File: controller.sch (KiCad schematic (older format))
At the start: 21 parts, among them J2 UART, J3 programming header, J4 Micro_SD_Card_Det, SW2 RAM~FLASH, SW3 start, SW4 stop, SW5 Rotary_Encoder_Switch, U1 WM8778-units, U5 STM32F401RC, U6 lcd, Y1 CSTLS4M00G53-B0

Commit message: ksch: change component values to include the unit except for resistors add more info to some devices
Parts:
- C31: value 4.7u -> 4.7uF
- C32: value 10u -> 10uF
- C33: value 0.1u -> 100nF
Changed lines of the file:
@@
 Sheet 3 4
 Title "OpenLoop"
-Date "2017-09-25"
+Date "2017-10-02"
 Rev "A"
 Comp ""
@@
 P 8900 5600
 F 0 "C33" H 8992 5646 50  0000 L CNN
-F 1 "0.1u" H 8992 5555 50  0000 L CNN
+F 1 "100nF" H 8992 5555 50  0000 L CNN
 F 2 "Capacitors_SMD:C_0805_HandSoldering" H 8900 5600 50  0001 C CNN
 F 3 "" H 8900 5600 50  0001 C CNN
@@
 P 7950 6150
 F 0 "C32" H 8100 6100 50  0000 R CNN
-F 1 "10u" H 8150 6200 50  0000 R CNN
+F 1 "10uF" H 8150 6200 50  0000 R CNN
 F 2 "Capacitors_SMD:C_0805_HandSoldering" H 7950 6150 50  0001 C CNN
 F 3 "" H 7950 6150 50  0001 C CNN
@@
 P 6950 4250
 F 0 "C31" H 7100 4200 50  0000 R CNN
-F 1 "4.7u" H 7150 4300 50  0000 R CNN
+F 1 "4.7uF" H 7150 4300 50  0000 R CNN
 F 2 "Capacitors_SMD:C_0805_HandSoldering" H 6950 4250 50  0001 C CNN
 F 3 "" H 6950 4250 50  0001 C CNN

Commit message: migrate to kicad v5
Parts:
- C31, C32, C33: symbol C_Small -> Device:C_Small
- J2: symbol CONN_01X02 -> Connector:Conn_01x02_Male
- J3: symbol CONN_01X04 -> Connector:Conn_01x04_Male
- J4: symbol Micro_SD_Card_Det -> Connector:Micro_SD_Card_Det
- R4, R5, R6, R7: symbol R_Small -> Device:R_Small
- RV1, RV2, RV3: symbol POT -> Device:R_POT
- SW2: symbol SW_SPDT -> Switch:SW_SPDT
- SW3, SW4: symbol SW_Push -> Switch:SW_Push
- SW5: symbol Rotary_Encoder_Switch -> Device:Rotary_Encoder_Switch
- U1: symbol WM8778-units -> openloop:WM8778-units
- U5: symbol STM32F401RC -> openloop:STM32F401RC
- U6: symbol lcd -> openloop:lcd
- Y1: symbol Resonator_Small -> Device:Resonator_Small
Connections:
- wire segments 60 -> 73
- no-connect marks 0 -> 21

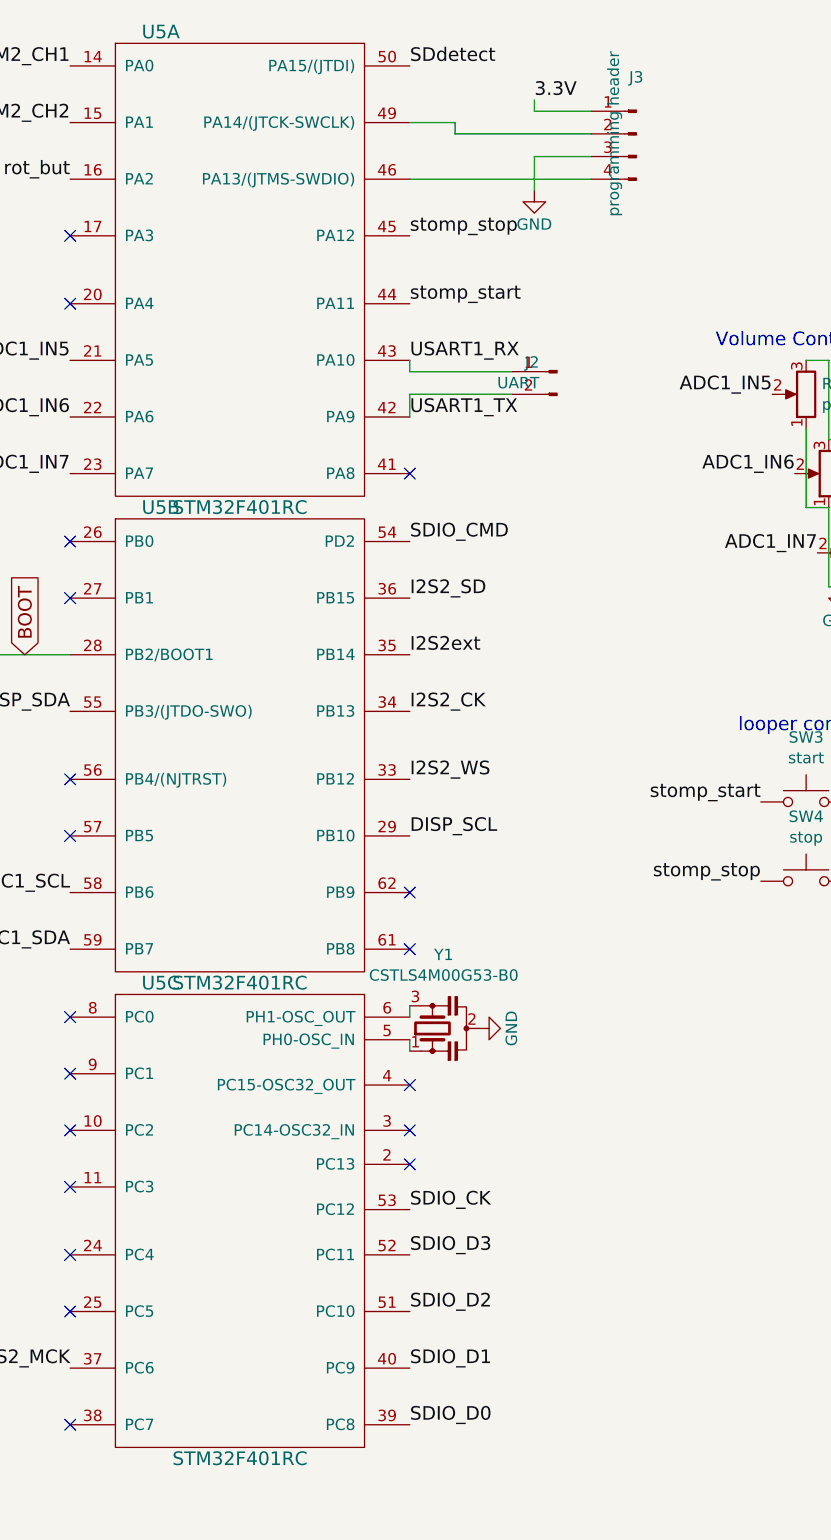
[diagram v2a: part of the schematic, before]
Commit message: ready for print
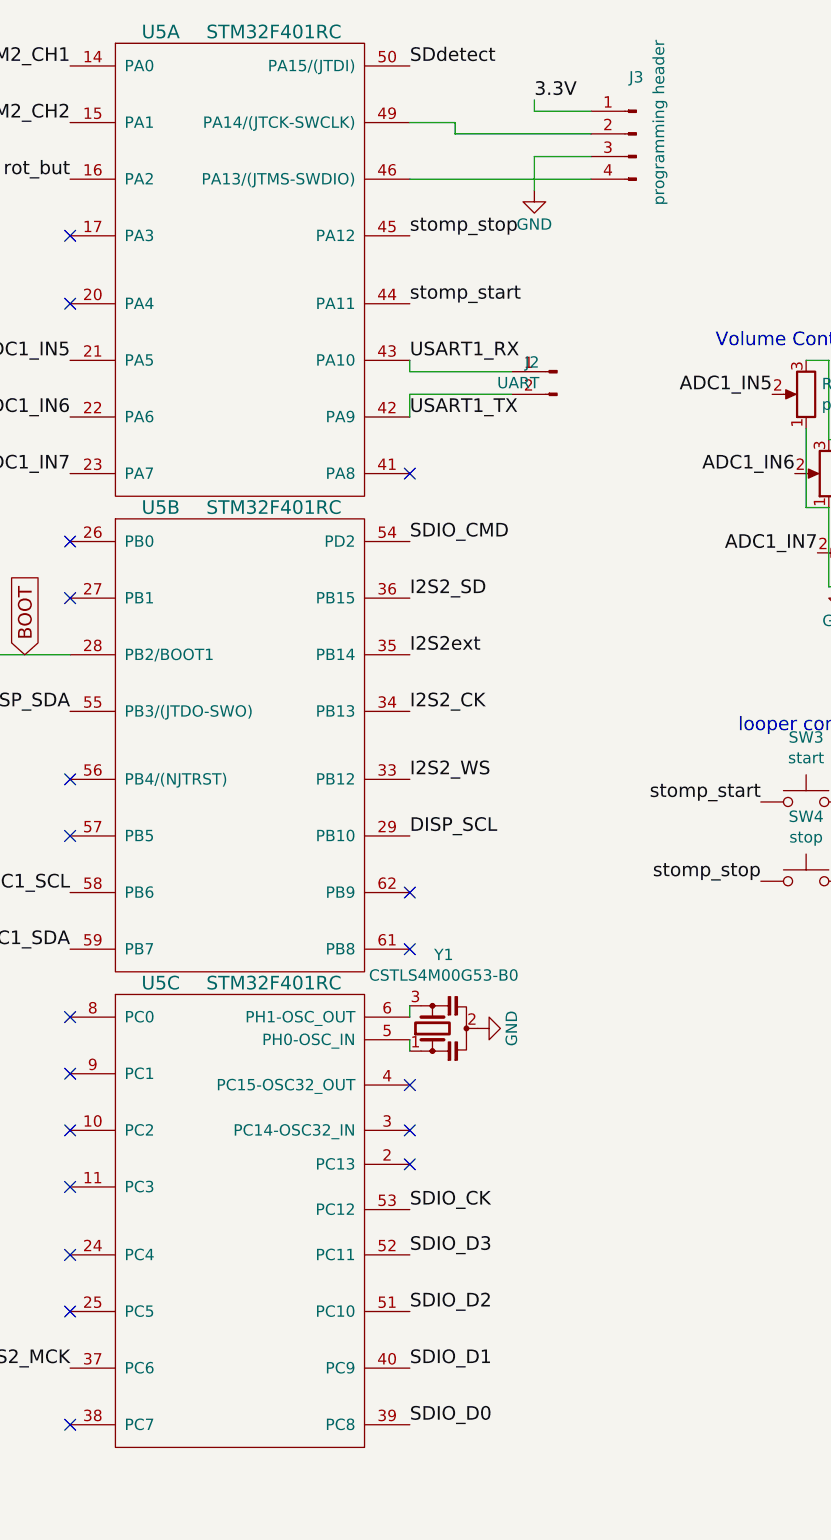
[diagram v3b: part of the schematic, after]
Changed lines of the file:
@@
 Sheet 3 4
 Title "OpenLoop"
-Date "2017-10-02"
+Date "2018-06-20"
 Rev "A"
 Comp ""
@@
 P 2550 1600
 F 0 "U5" H 2200 2650 60  0000 C CNN
-F 1 "STM32F401RC" H 2550 550 60  0000 C CNN
+F 1 "STM32F401RC" H 2700 2650 60  0000 C CNN
 F 2 "footprints:LQFP-64_10x10mm_Pitch0.5mm_HandSolder" H 2500 1550 60  0001 C CNN
 F 3 "" H 2500 1550 60  0001 C CNN
@@
 P 4300 1000
 F 0 "J3" H 4300 1250 50  0000 C CNN
-F 1 "programming header" V 4400 1000 50  0000 C CNN
+F 1 "programming header" V 4200 1050 50  0000 C CNN
 F 2 "Pin_Headers:Pin_Header_Straight_1x04_Pitch2.54mm" H 4300 1000 50  0001 C CNN
 F 3 "" H 4300 1000 50  0001 C CNN
@@
 P 2550 5800
 F 0 "U5" H 2200 6850 60  0000 C CNN
-F 1 "STM32F401RC" H 2550 4750 60  0000 C CNN
+F 1 "STM32F401RC" H 2700 6850 60  0000 C CNN
 F 2 "footprints:LQFP-64_10x10mm_Pitch0.5mm_HandSolder" H 2500 5750 60  0001 C CNN
 F 3 "" H 2500 5750 60  0001 C CNN
@@
 P 2550 3700
 F 0 "U5" H 2200 4750 60  0000 C CNN
-F 1 "STM32F401RC" H 2550 2650 60  0000 C CNN
+F 1 "STM32F401RC" H 2700 4750 60  0000 C CNN
 F 2 "footprints:LQFP-64_10x10mm_Pitch0.5mm_HandSolder" H 2500 3650 60  0001 C CNN
 F 3 "" H 2500 3650 60  0001 C CNN
